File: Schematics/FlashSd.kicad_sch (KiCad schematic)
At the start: 3 parts, among them J8 Micro_SD_Card

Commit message: output files got quote
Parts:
- J8: LCSC (none) -> C164170; LCSC Part C164170 -> (none)
- R15: LCSC (none) -> C84376; LCSC Part C84376 -> (none)
- R16: LCSC (none) -> C17557; LCSC Part C17557 -> (none)
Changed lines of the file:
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@@
-			)
-		)
-		(property "LCSC Part" "C84376"
-			(at 148.59 91.44 90)
-			(effects
-				(font
-					(size 1.27 1.27)
-				)
-				(hide yes)
 			)
 		)
@@
 		)
 		(property "Purchase-URL" ""
+			(at 148.59 91.44 90)
+			(effects
+				(font
+					(size 1.27 1.27)
+				)
+				(hide yes)
+			)
+		)
+		(property "LCSC" "C84376"
 			(at 148.59 91.44 90)
 			(effects
@@
 			)
 		)
-		(property "LCSC Part" "C17557"
-			(at 148.59 99.06 90)
-			(effects
-				(font
-					(size 1.27 1.27)
-				)
-				(hide yes)
-			)
-		)
 		(property "Description_1" ""
 			(at 148.59 99.06 90)
@@
 		)
 		(property "Purchase-URL" ""
+			(at 148.59 99.06 90)
+			(effects
+				(font
+					(size 1.27 1.27)
+				)
+				(hide yes)
+			)
+		)
+		(property "LCSC" "C17557"
 			(at 148.59 99.06 90)
 			(effects
@@
 			)
 		)
-		(property "LCSC Part" "C164170"
-			(at 194.31 96.52 0)
-			(effects
-				(font
-					(size 1.27 1.27)
-				)
-				(hide yes)
-			)
-		)
 		(property "Description_1" ""
 			(at 194.31 96.52 0)
@@
 			(at 194.31 96.52 0)
 			(effects
+				(font
+					(size 1.27 1.27)
+				)
+				(hide yes)
+			)
+		)
+		(property "LCSC" "C164170"
+			(at 194.31 96.52 0)
+			(effects

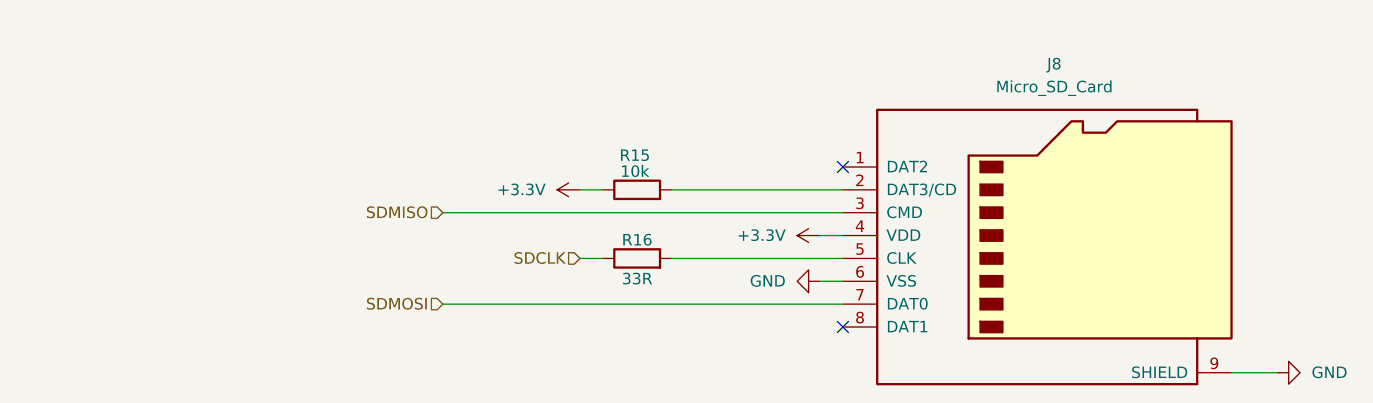
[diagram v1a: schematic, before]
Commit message: finalized output files
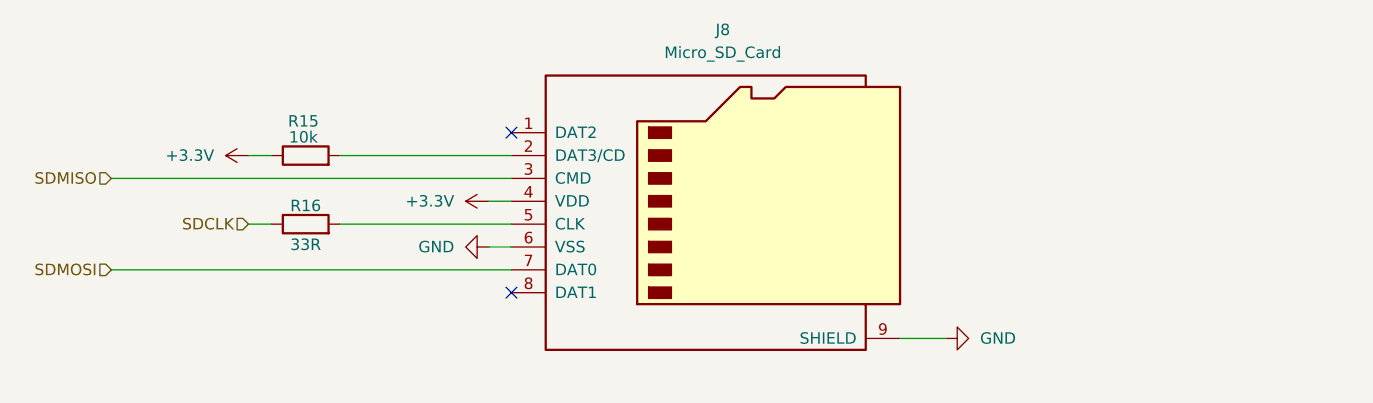
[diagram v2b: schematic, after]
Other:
- moved on the sheet: J8, R15, R16
